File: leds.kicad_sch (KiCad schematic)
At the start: 11 parts, among them IC1 STPIC6D595TTR, IC2 STPIC6D595TTR, IC3 STPIC6D595TTR, IC4 STPIC6D595TTR, IC5 STPIC6D595TTR

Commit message: New template
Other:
- company: (none) -> STAPsystem
- title: (none) -> RPM meter LED
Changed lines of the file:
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@@
 	(generator_version "8.0")
 	(paper "A3")
+	(title_block
+		(title "RPM meter LED")
+		(date "2024-11-26")
+		(rev "v1.0")
+		(company "STAPsystem")
+	)
 	(wire
 		(pts

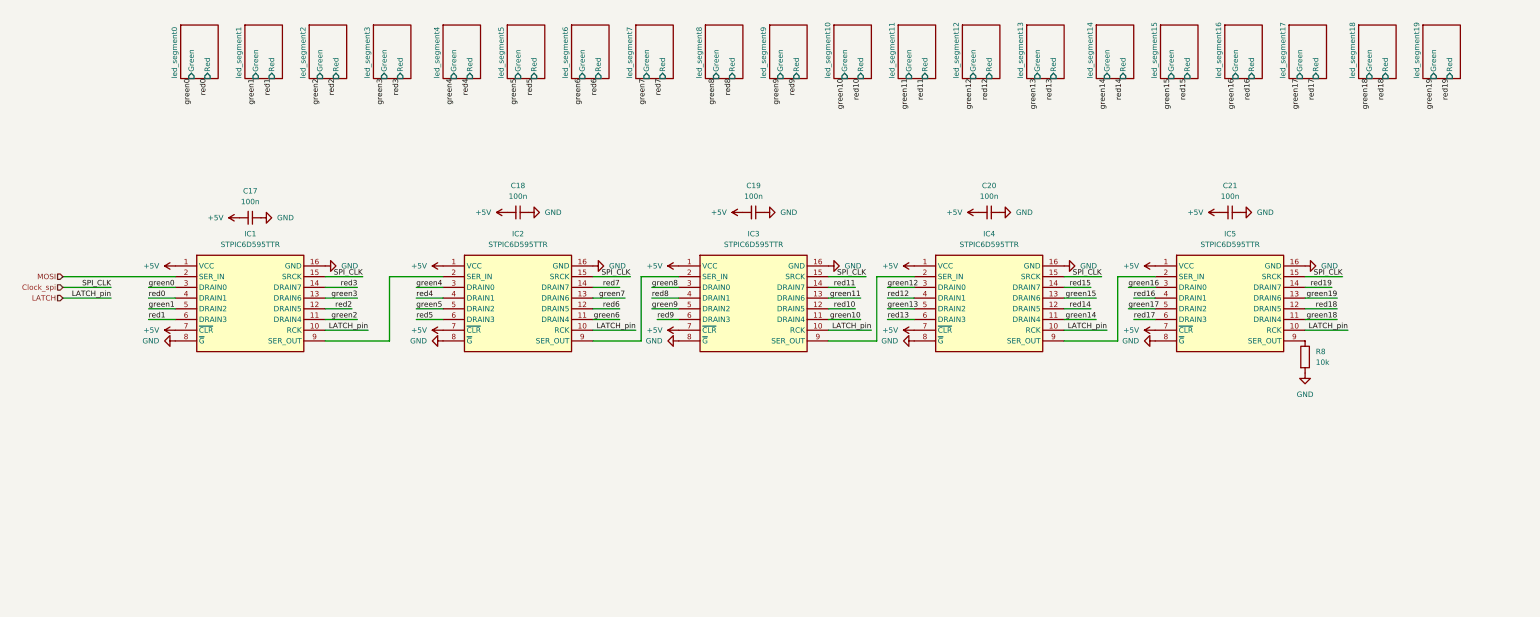
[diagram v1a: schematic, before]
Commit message: ws2812b
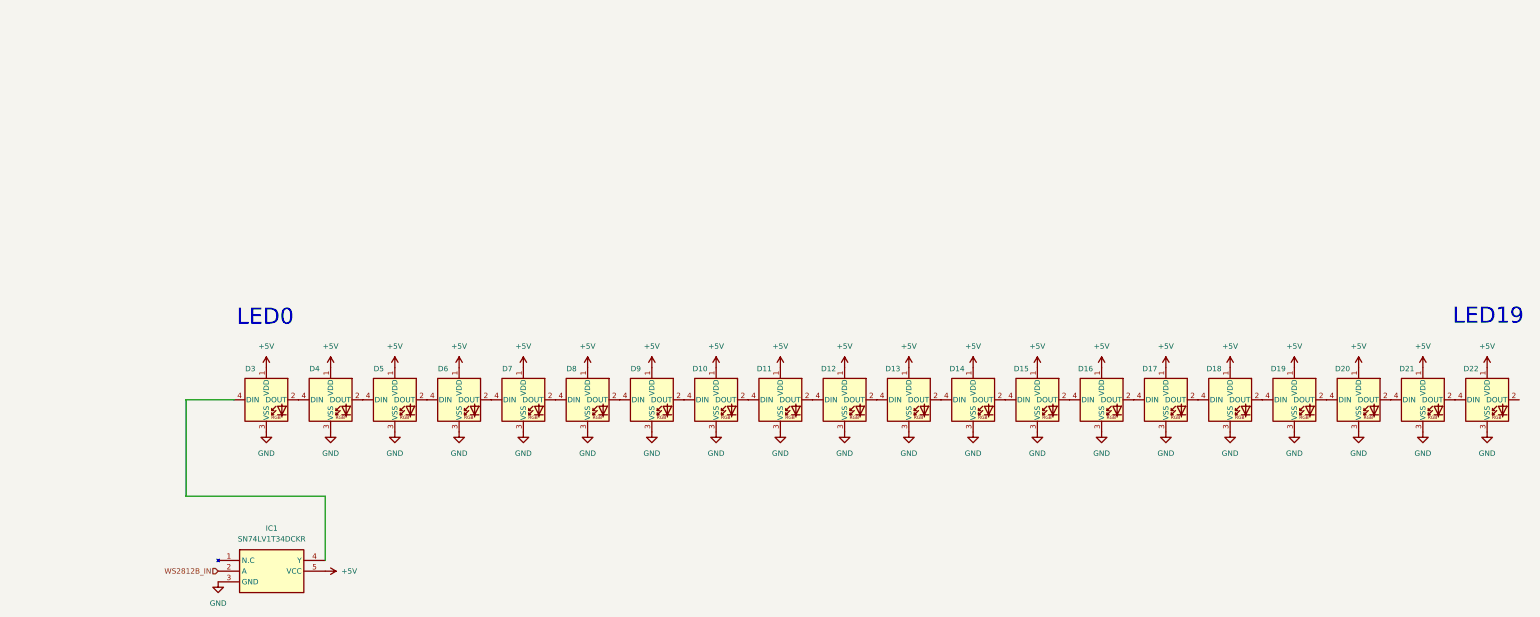
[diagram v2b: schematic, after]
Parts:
- removed C17, C18, C19, C20, C21: 100n, Capacitor_SMD:C_0603_1608Metric, symbol Device:C_Small
- removed IC1, IC2, IC3, IC4, IC5: STPIC6D595TTR, Library_local:SOP65P640X120-16N, symbol local_library:STPIC6D595TTR
- removed R8: 10k, Resistor_SMD:R_0603_1608Metric, symbol Device:R
- added D10, D11, D12, D13, D14, D15, D16, D17, D18, D19, D20, D21, D22, D3, D4, D5, D6, D7, D8, D9: WS2812B, LED_SMD:LED_WS2812B_PLCC4_5.0x5.0mm_P3.2mm, symbol LED:WS2812B
- added IC1: SN74LV1T34DCKR, Library_local:SOT65P210X110-5N, symbol local_library:SN74LV1T34DCKR
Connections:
- net +5V: now also D10.1 (VDD), D11.1 (VDD), D12.1 (VDD), D13.1 (VDD), D14.1 (VDD), D15.1 (VDD), D16.1 (VDD), D17.1 (VDD), D18.1 (VDD), D19.1 (VDD), D20.1 (VDD), D21.1 (VDD), D22.1 (VDD), D3.1 (VDD), D4.1 (VDD), D5.1 (VDD), D6.1 (VDD), D7.1 (VDD), D8.1 (VDD), D9.1 (VDD), IC1.5 (VCC)
- net GND: now also D10.3 (VSS), D11.3 (VSS), D12.3 (VSS), D13.3 (VSS), D14.3 (VSS), D15.3 (VSS), D16.3 (VSS), D17.3 (VSS), D18.3 (VSS), D19.3 (VSS), D20.3 (VSS), D21.3 (VSS), D22.3 (VSS), D3.3 (VSS), D4.3 (VSS), D5.3 (VSS), D6.3 (VSS), D7.3 (VSS), D8.3 (VSS), D9.3 (VSS), IC1.3 (GND)
- new net: D7.2 (DOUT), D8.4 (DIN)
- new net: D6.2 (DOUT), D7.4 (DIN)
- new net: D10.2 (DOUT), D11.4 (DIN)
- new net: D10.4 (DIN), D9.2 (DOUT)
- new net: D14.2 (DOUT), D15.4 (DIN)
- new net: D13.2 (DOUT), D14.4 (DIN)
- new net: D18.2 (DOUT), D19.4 (DIN)
- new net: D17.2 (DOUT), D18.4 (DIN)
- new net: D16.2 (DOUT), D17.4 (DIN)
- new net: D15.2 (DOUT), D16.4 (DIN)
- new net: D8.2 (DOUT), D9.4 (DIN)
- new net: D11.2 (DOUT), D12.4 (DIN)
- new net: D21.2 (DOUT), D22.4 (DIN)
- new net: D4.2 (DOUT), D5.4 (DIN)
- new net: D3.2 (DOUT), D4.4 (DIN)
- new net: D3.4 (DIN), IC1.4 (Y)
- new net: D12.2 (DOUT), D13.4 (DIN)
- new net: D19.2 (DOUT), D20.4 (DIN)
- new net: D5.2 (DOUT), D6.4 (DIN)
- new net: D20.2 (DOUT), D21.4 (DIN)
- new net WS2812B_IN: IC1.2 (A)
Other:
- removed sheet led_segment0
- removed sheet led_segment1
- removed sheet led_segment10
- removed sheet led_segment11
- removed sheet led_segment12
- removed sheet led_segment13
- removed sheet led_segment14
- removed sheet led_segment15
- removed sheet led_segment16
- removed sheet led_segment17
- removed sheet led_segment18
- removed sheet led_segment19
- removed sheet led_segment2
- removed sheet led_segment3
- removed sheet led_segment4
- removed sheet led_segment5
- removed sheet led_segment6
- removed sheet led_segment7
- removed sheet led_segment8
- removed sheet led_segment9
- note added: "LED0"
- note added: "LED19"
